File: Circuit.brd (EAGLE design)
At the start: 99 x 72.1 mm, 115 parts, among them IC1 LM1117T-3.3-V, P1 RASPI-P1RASPI_REV2_P1, P5 RASPI_P5

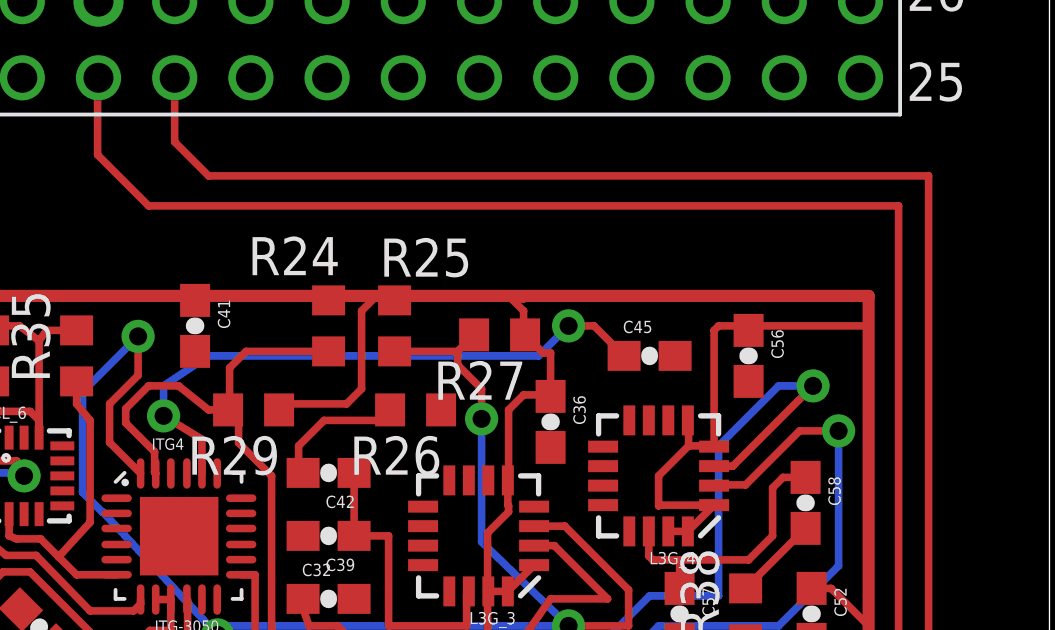
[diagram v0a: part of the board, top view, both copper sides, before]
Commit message: Pause before Skins. I think I've got all airwires?
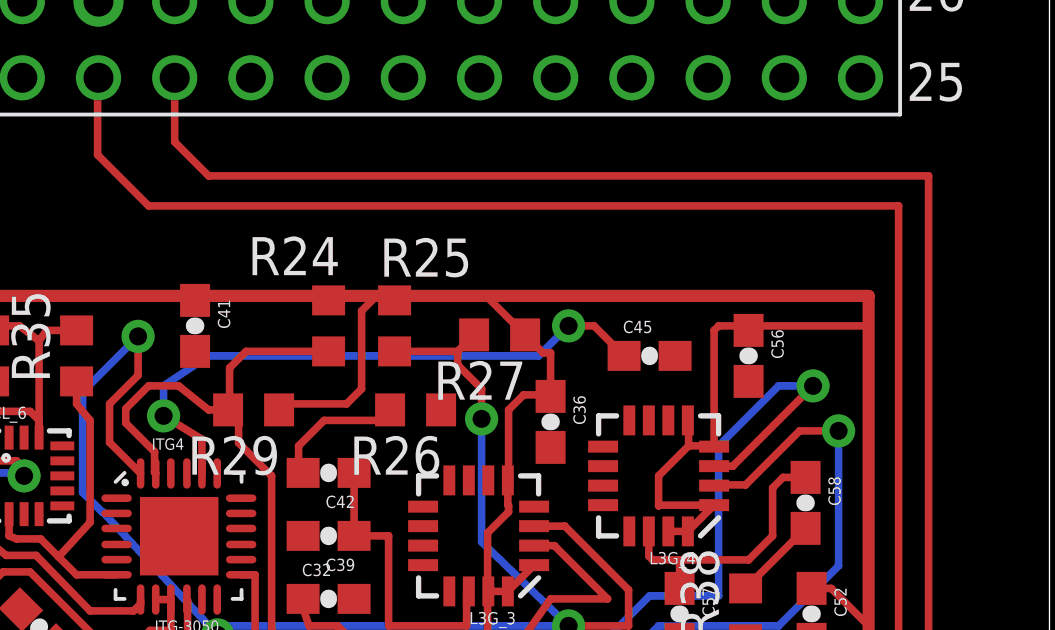
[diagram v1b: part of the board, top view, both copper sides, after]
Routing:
- net +3V3: track 702.8 -> 691.9 mm
- net N$4: track 3.03 -> 0.00 mm
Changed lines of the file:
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@@
 <wire x1="93" y1="29" x2="93" y2="39" width="0.254" layer="1"/>
 <wire x1="93" y1="39" x2="93" y2="40" width="0.254" layer="1"/>
-<wire x1="93" y1="40" x2="77" y2="40" width="0.254" layer="1"/>
 <wire x1="76.6" y1="40" x2="75" y2="40" width="0.254" layer="1"/>
 <wire x1="75" y1="40" x2="70.25" y2="40" width="0.254" layer="1"/>
@@
 <wire x1="29.85" y1="21.1" x2="30.1" y2="20.9" width="0.254" layer="1"/>
 <wire x1="30.1" y1="20.9" x2="30" y2="21" width="0.254" layer="1"/>
-<wire x1="93" y1="40" x2="70.25" y2="40" width="0.4064" layer="1"/>
+<wire x1="93" y1="40" x2="77" y2="40" width="0.4064" layer="1"/>
+<wire x1="77" y1="40" x2="70.25" y2="40" width="0.4064" layer="1"/>
 <wire x1="70.25" y1="40" x2="63.8" y2="40" width="0.4064" layer="1"/>
 <wire x1="63.8" y1="40" x2="61" y2="40" width="0.4064" layer="1"/>
@@
 <wire x1="72.75" y1="27.9" x2="72.75" y2="26.75" width="0.254" layer="16"/>
 <wire x1="72.75" y1="26.75" x2="72" y2="26" width="0.254" layer="16"/>
+<wire x1="77" y1="40" x2="80.25" y2="40" width="0.254" layer="1"/>
+<wire x1="80.25" y1="40" x2="81.55" y2="38.7" width="0.254" layer="1"/>
 <wire x1="89" y1="39" x2="89" y2="38.85" width="0" layer="19" extent="1-1"/>
 <wire x1="34.75" y1="18.25" x2="34.6" y2="18.25" width="0" layer="19" extent="1-1"/>
-<wire x1="74" y1="30" x2="72.55" y2="30.7033" width="0" layer="19" extent="1-1"/>
 <wire x1="36.6" y1="39.85" x2="34.3" y2="39.85" width="0" layer="19" extent="1-1"/>
 </signal>
@@
 </signal>
 <signal name="N$4">
-<wire x1="81.5" y1="39.9" x2="81.45" y2="39.95" width="0.254" layer="1"/>
-<wire x1="81.5" y1="38.65" x2="81.5" y2="39.5" width="0.254" layer="1"/>
-<wire x1="81.5" y1="39.5" x2="81.1" y2="39.9" width="0.254" layer="1"/>
-<wire x1="82" y1="40" x2="81" y2="40" width="0.254" layer="1"/>
-<wire x1="81.5" y1="39.9" x2="81.1" y2="39.9" width="0.254" layer="1"/>
-<wire x1="81.1" y1="39.9" x2="81" y2="40" width="0.254" layer="1"/>
 </signal>
 </signals>
